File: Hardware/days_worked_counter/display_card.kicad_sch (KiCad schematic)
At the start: 28 parts, among them J501 Top Conn, J502 Bottom Conn, Q501 MMBT3904, Q502 MMBT3904, Q503 MMBT3904, Q504 MMBT3904, Q505 MMBT3904, Q506 MMBT3904, Q507 MMBT3904, Q508 MMBT3904, U501 SN74HC595

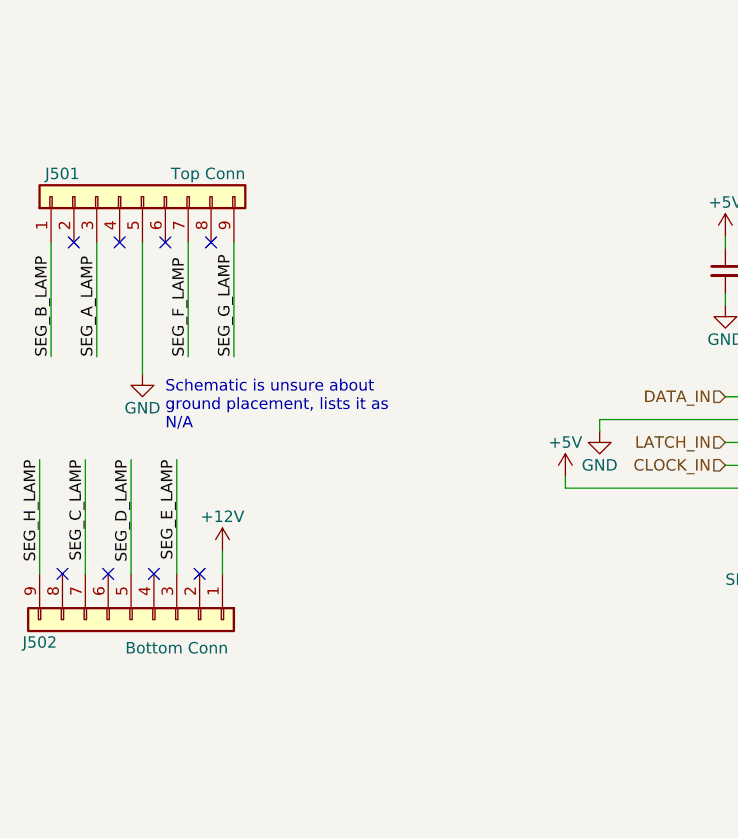
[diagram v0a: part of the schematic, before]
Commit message: Add stuff
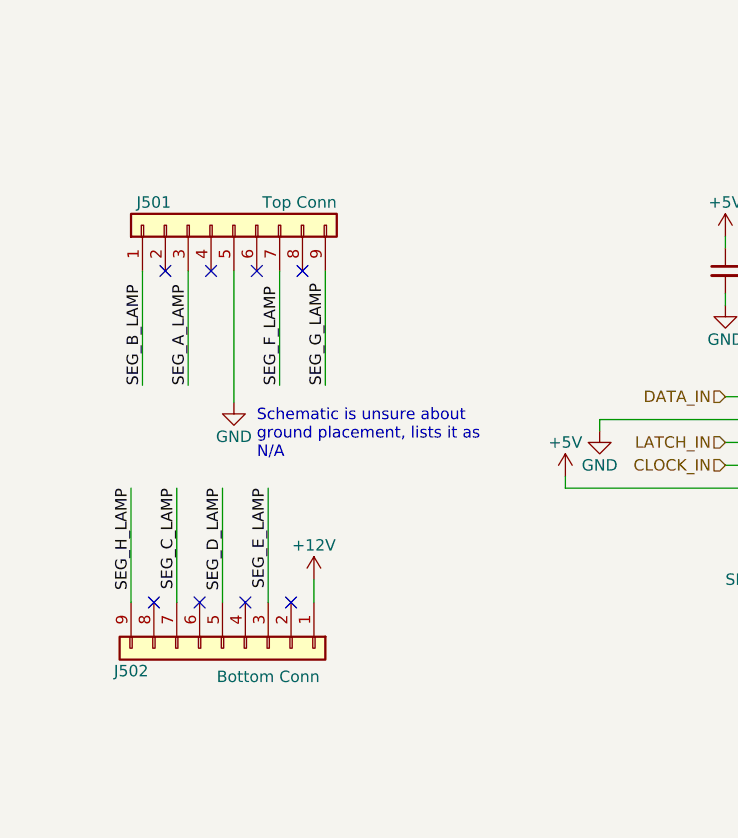
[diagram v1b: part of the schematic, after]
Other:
- moved on the sheet: J501, J502
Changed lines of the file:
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@@
   (junction (at 255.27 93.98) (diameter 0) (color 0 0 0 0)
   )
-  (no_connect (at 69.85 73.025))
-  (no_connect (at 74.93 73.025))
-  (no_connect (at 59.69 73.025))
-  (no_connect (at 58.42 109.855))
-  (no_connect (at 68.58 109.855))
-  (no_connect (at 63.5 109.855))
-  (no_connect (at 73.66 109.855))
-  (no_connect (at 64.77 73.025))
+  (no_connect (at 80.01 76.2))
+  (no_connect (at 85.09 76.2))
+  (no_connect (at 69.85 76.2))
+  (no_connect (at 68.58 113.03))
+  (no_connect (at 78.74 113.03))
+  (no_connect (at 73.66 113.03))
+  (no_connect (at 83.82 113.03))
+  (no_connect (at 74.93 76.2))
   (wire (pts (xy 242.57 19.05) (xy 229.87 19.05))
     (stroke (width 0) (type default) (color 0 0 0 0))
@@
     (stroke (width 0) (type default) (color 0 0 0 0))
   )
-  (wire (pts (xy 77.47 85.725) (xy 77.47 73.025))
+  (wire (pts (xy 87.63 88.9) (xy 87.63 76.2))
     (stroke (width 0) (type default) (color 0 0 0 0))
   )
@@
     (stroke (width 0) (type default) (color 0 0 0 0))
   )
-  (wire (pts (xy 55.88 97.155) (xy 55.88 109.855))
+  (wire (pts (xy 66.04 100.33) (xy 66.04 113.03))
     (stroke (width 0) (type default) (color 0 0 0 0))
   )
@@
     (stroke (width 0) (type default) (color 0 0 0 0))
   )
-  (wire (pts (xy 57.15 85.725) (xy 57.15 73.025))
+  (wire (pts (xy 67.31 88.9) (xy 67.31 76.2))
     (stroke (width 0) (type default) (color 0 0 0 0))
   )
@@
     (stroke (width 0) (type default) (color 0 0 0 0))
   )
-  (wire (pts (xy 71.12 97.155) (xy 71.12 109.855))
+  (wire (pts (xy 81.28 100.33) (xy 81.28 113.03))
     (stroke (width 0) (type default) (color 0 0 0 0))
   )
@@
     (stroke (width 0) (type default) (color 0 0 0 0))
   )
-  (wire (pts (xy 62.23 85.725) (xy 62.23 73.025))
+  (wire (pts (xy 72.39 88.9) (xy 72.39 76.2))
     (stroke (width 0) (type default) (color 0 0 0 0))
   )
@@
     (stroke (width 0) (type default) (color 0 0 0 0))
   )
-  (wire (pts (xy 67.31 87.63) (xy 67.31 73.025))
+  (wire (pts (xy 77.47 90.805) (xy 77.47 76.2))
     (stroke (width 0) (type default) (color 0 0 0 0))
   )
@@
     (stroke (width 0) (type default) (color 0 0 0 0))
   )
-  (wire (pts (xy 60.96 97.155) (xy 60.96 109.855))
+  (wire (pts (xy 71.12 100.33) (xy 71.12 113.03))
     (stroke (width 0) (type default) (color 0 0 0 0))
   )
@@
     (stroke (width 0) (type default) (color 0 0 0 0))
   )
-  (wire (pts (xy 66.04 97.155) (xy 66.04 109.855))
+  (wire (pts (xy 76.2 100.33) (xy 76.2 113.03))
     (stroke (width 0) (type default) (color 0 0 0 0))
   )
@@
     (stroke (width 0) (type default) (color 0 0 0 0))
   )
-  (wire (pts (xy 72.39 85.725) (xy 72.39 73.025))
+  (wire (pts (xy 82.55 88.9) (xy 82.55 76.2))
     (stroke (width 0) (type default) (color 0 0 0 0))
   )
@@
     (stroke (width 0) (type default) (color 0 0 0 0))
   )
-  (wire (pts (xy 76.2 107.315) (xy 76.2 109.855))
+  (wire (pts (xy 86.36 110.49) (xy 86.36 113.03))
     (stroke (width 0) (type default) (color 0 0 0 0))
   )
@@
   )
   (text "Schematic is unsure about\nground placement, lists it as\nN/A"
-    (at 69.85 93.98 0)
+    (at 80.01 97.155 0)
     (effects (font (size 1.27 1.27)) (justify left bottom))
   )
@@
     (effects (font (size 1.27 1.27)) (justify right bottom))
   )
-  (label "SEG_B_LAMP" (at 57.15 85.725 90)
+  (label "SEG_B_LAMP" (at 67.31 88.9 90)
     (effects (font (size 1.27 1.27)) (justify left bottom))
   )
@@
     (effects (font (size 1.27 1.27)) (justify right bottom))
   )
-  (label "SEG_A_LAMP" (at 62.23 85.725 90)
+  (label "SEG_A_LAMP" (at 72.39 88.9 90)
     (effects (font (size 1.27 1.27)) (justify left bottom))
   )
@@
     (effects (font (size 1.27 1.27)) (justify right bottom))
   )
-  (label "SEG_D_LAMP" (at 66.04 97.155 270)
+  (label "SEG_D_LAMP" (at 76.2 100.33 270)
     (effects (font (size 1.27 1.27)) (justify right bottom))
   )
@@
     (effects (font (size 1.27 1.27)) (justify right bottom))
   )
-  (label "SEG_E_LAMP" (at 71.12 97.155 270)
+  (label "SEG_E_LAMP" (at 81.28 100.33 270)
     (effects (font (size 1.27 1.27)) (justify right bottom))
   )
@@
     (effects (font (size 1.27 1.27)) (justify left bottom))
   )
-  (label "SEG_F_LAMP" (at 72.39 85.725 90)
+  (label "SEG_F_LAMP" (at 82.55 88.9 90)
     (effects (font (size 1.27 1.27)) (justify left bottom))
   )
@@
     (effects (font (size 1.27 1.27)) (justify right bottom))
   )
-  (label "SEG_H_LAMP" (at 55.88 97.155 270)
+  (label "SEG_H_LAMP" (at 66.04 100.33 270)
     (effects (font (size 1.27 1.27)) (justify right bottom))
   )
@@
     (effects (font (size 1.27 1.27)) (justify left bottom))
   )
-  (label "SEG_G_LAMP" (at 77.47 85.725 90)
+  (label "SEG_G_LAMP" (at 87.63 88.9 90)
     (effects (font (size 1.27 1.27)) (justify left bottom))
   )
@@
     (effects (font (size 1.27 1.27)) (justify left bottom))
   )
-  (label "SEG_C_LAMP" (at 60.96 97.155 270)
+  (label "SEG_C_LAMP" (at 71.12 100.33 270)
     (effects (font (size 1.27 1.27)) (justify right bottom))
   )
@@
     (effects (font (size 1.27 1.27)) (justify left))
   )
-  (symbol (lib_id "power:+12V") (at 76.2 107.315 0) (unit 1)
-    (in_bom yes) (on_board yes)
-    (property "Reference" "#PWR0151" (id 0) (at 76.2 111.125 0)
-      (effects (font (size 1.27 1.27)) hide)
-    )
-    (property "Value" "+12V" (id 1) (at 76.2 103.505 0))
-    (property "Footprint" "" (id 2) (at 76.2 107.315 0)
-      (effects (font (size 1.27 1.27)) hide)
-    )
-    (property "Datasheet" "" (id 3) (at 76.2 107.315 0)
+  (symbol (lib_id "power:+12V") (at 86.36 110.49 0) (unit 1)
+    (in_bom yes) (on_board yes)
+    (property "Reference" "#PWR0151" (id 0) (at 86.36 114.3 0)
+      (effects (font (size 1.27 1.27)) hide)
+    )
+    (property "Value" "+12V" (id 1) (at 86.36 106.68 0))
+    (property "Footprint" "" (id 2) (at 86.36 110.49 0)
+      (effects (font (size 1.27 1.27)) hide)
+    )
+    (property "Datasheet" "" (id 3) (at 86.36 110.49 0)
       (effects (font (size 1.27 1.27)) hide)
     )
@@
     (pin "1")
   )
-  (symbol (lib_id "Connector_Generic:Conn_01x09") (at 67.31 67.945 90) (unit 1)
-    (in_bom yes) (on_board yes)
-    (property "Reference" "J501" (id 0) (at 60.325 65.405 90)
-      (effects (font (size 1.27 1.27)) (justify left))
-    )
-    (property "Value" "Top Conn" (id 1) (at 78.74 65.405 90)
-      (effects (font (size 1.27 1.27)) (justify left))
-    )
-    (property "Footprint" "Connector_PinSocket_2.54mm:PinSocket_1x09_P2.54mm_Vertical" (id 2) (at 67.31 67.945 0)
-      (effects (font (size 1.27 1.27)) hide)
-    )
-    (property "Datasheet" "~" (id 3) (at 67.31 67.945 0)
+  (symbol (lib_id "Connector_Generic:Conn_01x09") (at 77.47 71.12 90) (unit 1)
+    (in_bom yes) (on_board yes)
+    (property "Reference" "J501" (id 0) (at 70.485 68.58 90)
+      (effects (font (size 1.27 1.27)) (justify left))
+    )
+    (property "Value" "Top Conn" (id 1) (at 88.9 68.58 90)
+      (effects (font (size 1.27 1.27)) (justify left))
+    )
+    (property "Footprint" "Connector_PinSocket_2.54mm:PinSocket_1x09_P2.54mm_Vertical" (id 2) (at 77.47 71.12 0)
+      (effects (font (size 1.27 1.27)) hide)
+    )
+    (property "Datasheet" "~" (id 3) (at 77.47 71.12 0)
       (effects (font (size 1.27 1.27)) hide)
     )
@@
     (pin "2")
   )
-  (symbol (lib_id "power:GND") (at 67.31 87.63 0) (unit 1)
-    (in_bom yes) (on_board yes)
-    (property "Reference" "#PWR0150" (id 0) (at 67.31 93.98 0)
-      (effects (font (size 1.27 1.27)) hide)
-    )
-    (property "Value" "GND" (id 1) (at 67.31 91.44 0))
-    (property "Footprint" "" (id 2) (at 67.31 87.63 0)
-      (effects (font (size 1.27 1.27)) hide)
-    )
-    (property "Datasheet" "" (id 3) (at 67.31 87.63 0)
+  (symbol (lib_id "power:GND") (at 77.47 90.805 0) (unit 1)
+    (in_bom yes) (on_board yes)
+    (property "Reference" "#PWR0150" (id 0) (at 77.47 97.155 0)
+      (effects (font (size 1.27 1.27)) hide)
+    )
+    (property "Value" "GND" (id 1) (at 77.47 94.615 0))
+    (property "Footprint" "" (id 2) (at 77.47 90.805 0)
+      (effects (font (size 1.27 1.27)) hide)
+    )
+    (property "Datasheet" "" (id 3) (at 77.47 90.805 0)
       (effects (font (size 1.27 1.27)) hide)
     )
@@
     (pin "1")
   )
-  (symbol (lib_id "Connector_Generic:Conn_01x09") (at 66.04 114.935 270) (unit 1)
-    (in_bom yes) (on_board yes)
-    (property "Reference" "J502" (id 0) (at 53.975 117.475 90)
-      (effects (font (size 1.27 1.27)) (justify left))
-    )
-    (property "Value" "Bottom Conn" (id 1) (at 65.405 118.11 90)
-      (effects (font (size 1.27 1.27)) (justify left))
-    )
-    (property "Footprint" "Connector_PinSocket_2.54mm:PinSocket_1x09_P2.54mm_Vertical" (id 2) (at 66.04 114.935 0)
-      (effects (font (size 1.27 1.27)) hide)
-    )
-    (property "Datasheet" "~" (id 3) (at 66.04 114.935 0)
-      (effects (font (size 1.27 1.27)) hide)
-    )
+  (symbol (lib_id "Connector_Generic:Conn_01x09") (at 76.2 118.11 270) (unit 1)
+    (in_bom yes) (on_board yes)
+    (property "Reference" "J502" (id 0) (at 64.135 120.65 90)
+      (effects (font (size 1.27 1.27)) (justify left))
+    )
+    (property "Value" "Bottom Conn" (id 1) (at 75.565 121.285 90)
+      (effects (font (size 1.27 1.27)) (justify left))
+    )
+    (property "Footprint" "Connector_PinSocket_2.54mm:PinSocket_1x09_P2.54mm_Vertical" (id 2) (at 76.2 118.11 0)
+      (effects (font (size 1.27 1.27)) hide)
+    )
+    (property "Datasheet" "~" (id 3) (at 76.2 118.11 0)
+      (effects (font (size 1.27 1.27)) hide)
+    )
